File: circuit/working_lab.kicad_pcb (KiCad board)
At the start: 2 copper layers, 13 parts, among them J1 Screw_Terminal_01x02, J2 UART, J3 PIC_KIT, J4 SPI, J5 I2C, U1 L7805, U2 PIC16F886-IP, Y1 2MHz

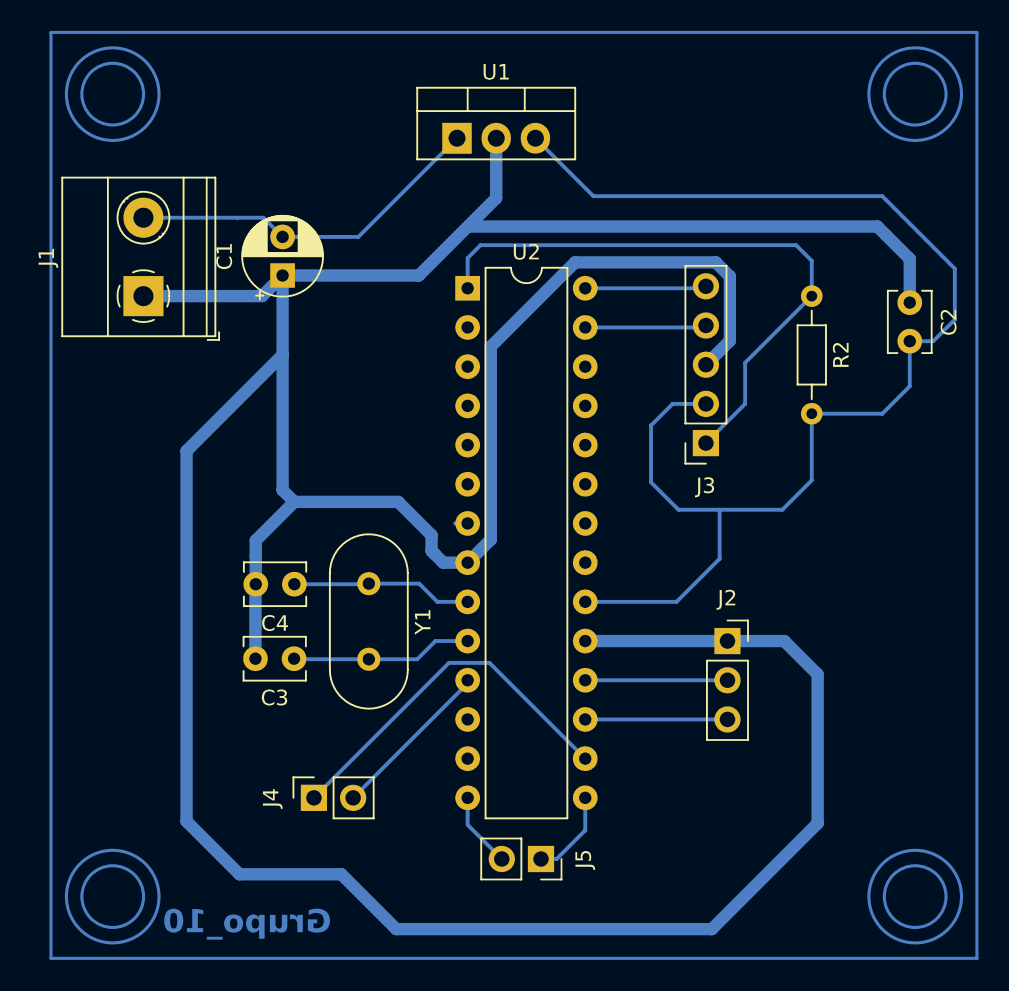
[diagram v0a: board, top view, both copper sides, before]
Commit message: circuit completed
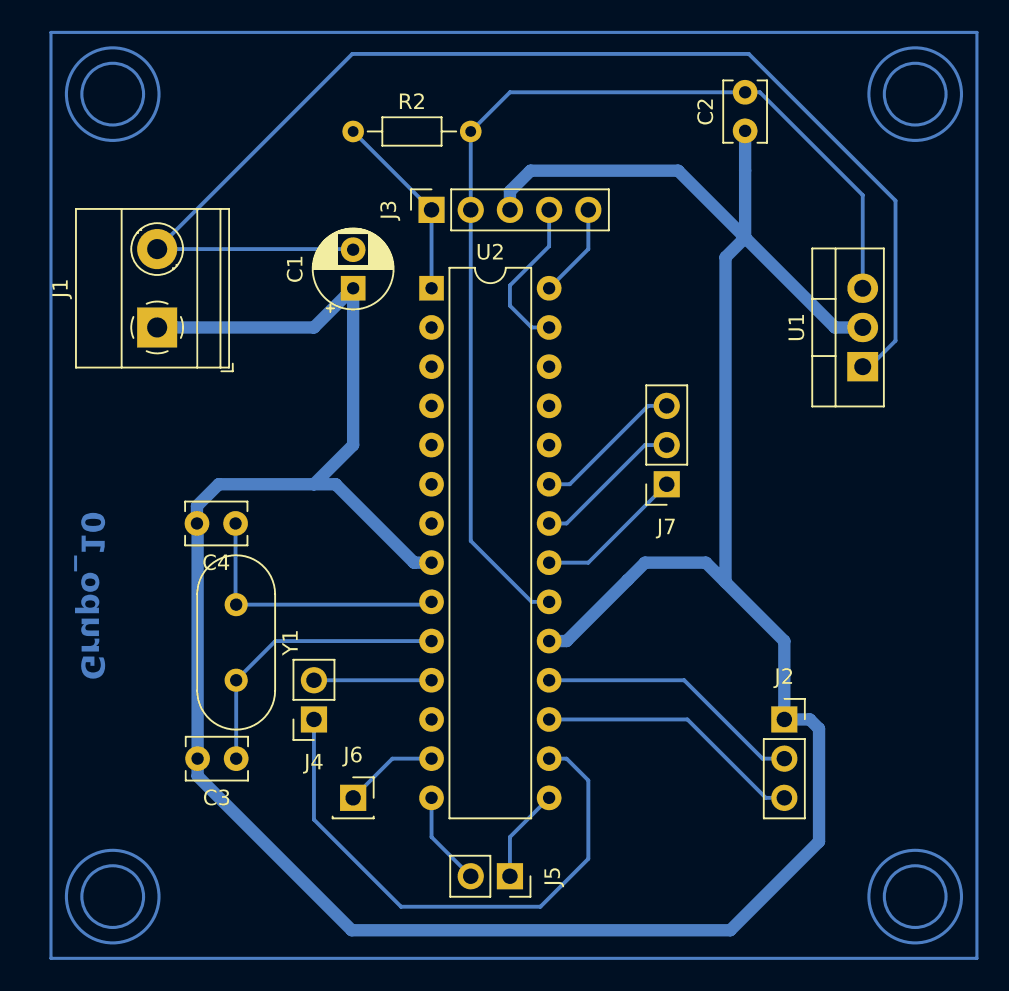
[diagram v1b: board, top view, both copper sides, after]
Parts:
- added J6: PWM, Connector_PinSocket_2.54mm:PinSocket_1x01_P2.54mm_Vertical, F.Cu at (68.6, 101.6)
- added J7: Analogic, Connector_PinSocket_2.54mm:PinSocket_1x03_P2.54mm_Vertical, F.Cu at (88.9, 81.3)
- moved R2 31.6 mm to (68.6, 58.4), turned to 0 degrees
- moved U1 30.2 mm to (101.6, 73.7), turned to 90 degrees
- moved J3 23.3 mm to (73.7, 63.5), turned to 90 degrees
- moved C2 15.4 mm to (94.0, 58.4), turned to 90 degrees
- moved Y1 8.70 mm to (61.0, 89.1)
- moved C3 7.48 mm to (61.0, 99.1)
- moved J2 6.27 mm to (96.5, 96.5)
- moved C4 5.48 mm to (61.0, 83.8)
- moved J4 5.08 mm to (66.0, 96.5), turned to 180 degrees
- moved C1 4.65 mm to (68.6, 68.6)
- moved U2 2.34 mm to (73.7, 68.6)
- moved J5 2.30 mm to (78.7, 106.7)
- moved J1 2.22 mm to (55.9, 71.1)
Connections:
- U2 pad 13: unconnected-(U2-RC2/P1A/CCP1-Pad13) -> Net-(J6-Pin_1)
- U2 pad 21: unconnected-(U2-INT/AN12/RB0-Pad21) -> Net-(J7-Pin_1)
- U2 pad 22: unconnected-(U2-P1C/AN10/RB1-Pad22) -> Net-(J7-Pin_2)
- U2 pad 23: unconnected-(U2-P1B/AN8/RB2-Pad23) -> Net-(J7-Pin_3)
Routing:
- net GND: track 288.5 -> 202.6 mm
- net +12V: track 23.5 -> 81.6 mm
- net mclr: track 39.7 -> 12.3 mm
- net VDD: track 84.6 -> 68.5 mm
- net dataOUT: track 23.8 -> 36.1 mm
- net Net-(J7-Pin_3): track 0.00 -> 9.72 mm
- net Net-(J7-Pin_2): track 0.00 -> 9.72 mm
- net Net-(J7-Pin_1): track 0.00 -> 9.72 mm
- net tx: track 9.22 -> 17.3 mm
- net rx: track 9.22 -> 17.3 mm
- net Net-(U2-CLKOUT/OSC2/RA6): track 11.8 -> 18.8 mm
- net Net-(U2-CLKIN/OSC1/RA7): track 11.7 -> 18.0 mm
- net Net-(J6-Pin_1): track 0.00 -> 6.13 mm
- net clk: track 10.7 -> 7.62 mm
- net ICSPCLK: track 7.87 -> 10.4 mm
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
